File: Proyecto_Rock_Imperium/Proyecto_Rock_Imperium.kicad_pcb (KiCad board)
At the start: 2 copper layers, 53.3 x 58.4 mm, 20 parts, among them Q1 2N3904, Q2 2N3904, SW1 SW_SPDT

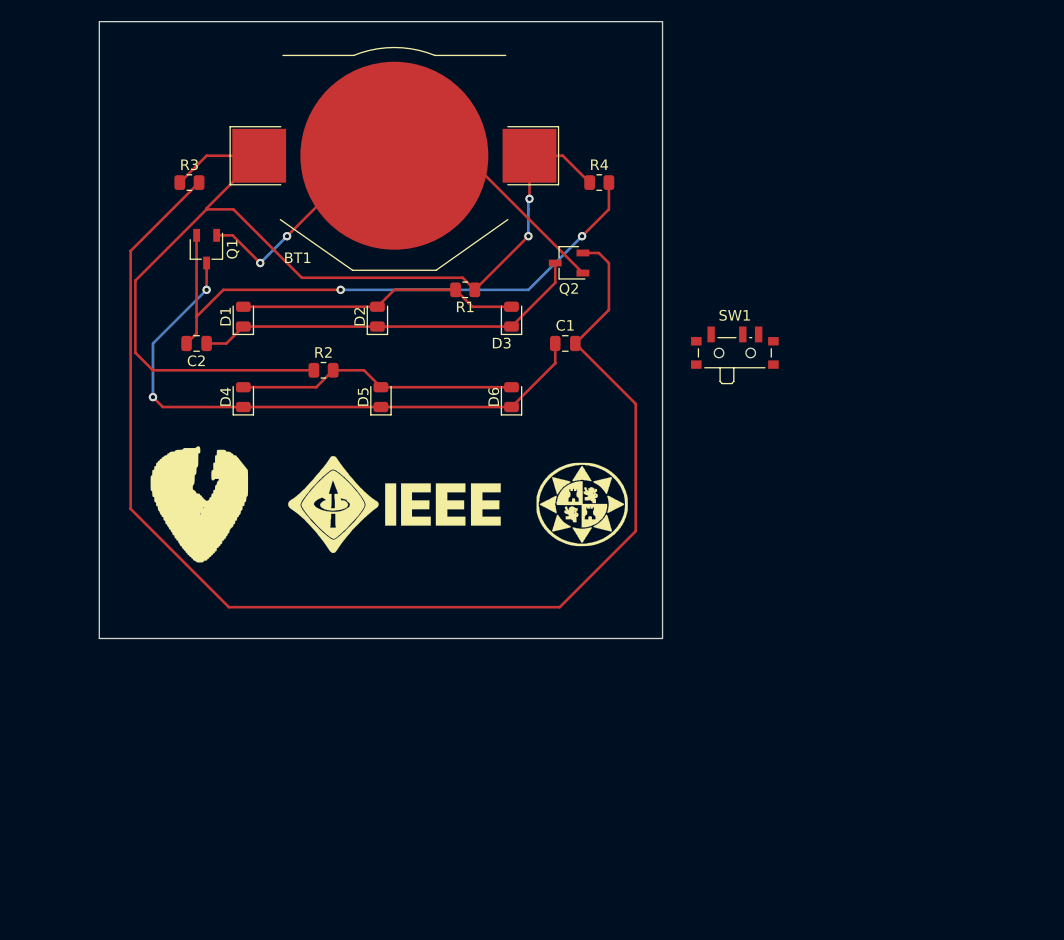
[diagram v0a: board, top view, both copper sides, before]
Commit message: terminado a falta de revision
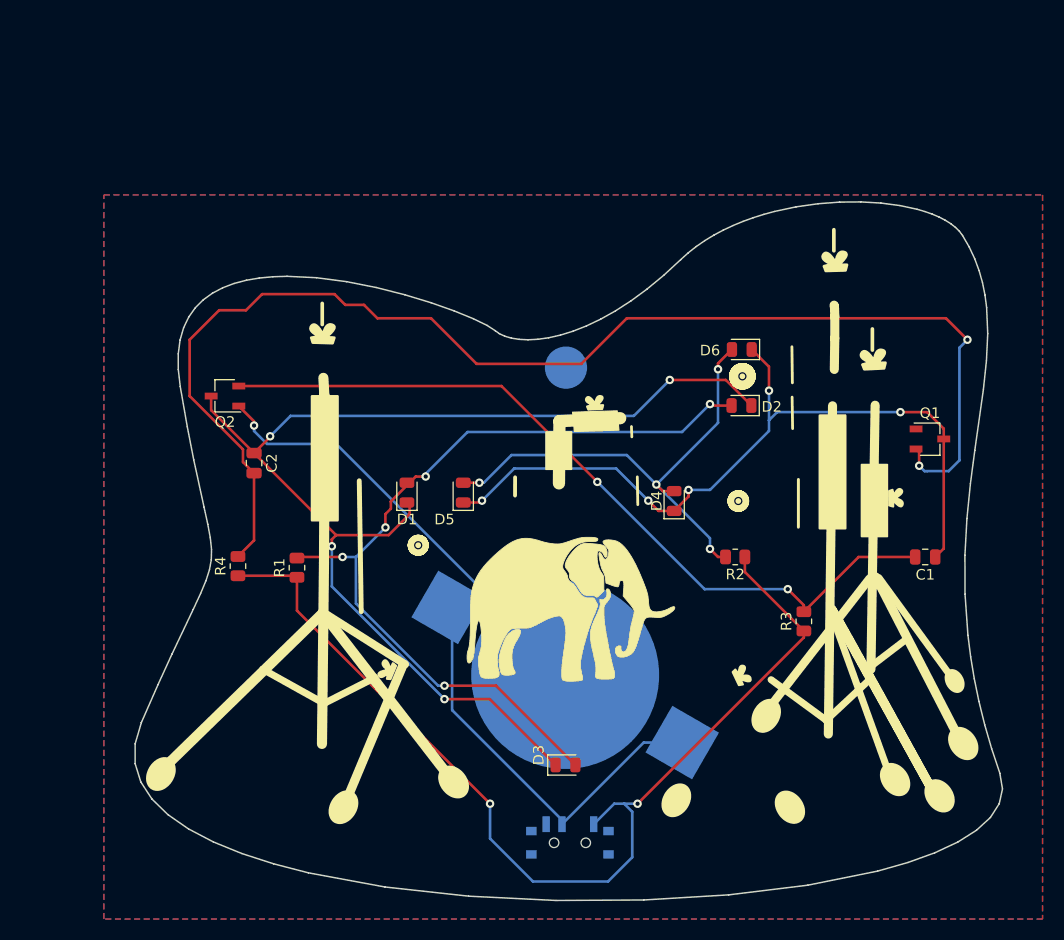
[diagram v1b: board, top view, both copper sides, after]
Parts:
- removed Ref**: Val**, proyecto_rock:RoCkImPeRiUm
- removed Ref**: Val**, proyecto_rock:IEEE2
- removed Ref**: Val**, proyecto_rock:UPCT2
- removed Ref**: Val**, proyecto_rock:UPCT
- added REF**: TestPoint_Pad_D4.0mm, TestPoint:TestPoint_Pad_D4.0mm, B.Cu at (156.0, 78.5)
- BT1, SW1: moved to B.Cu
- moved R3 71.5 mm to (178.5, 102.5), turned to 90 degrees
- moved Q1 70.8 mm to (190.4, 85.2), turned to 0 degrees
- moved BT1 51.8 mm to (155.9, 107.6), turned to 150 degrees
- moved R4 49.9 mm to (124.9, 97.3), turned to 90 degrees
- moved SW1 48.9 mm to (156.3, 123.2), turned to 180 degrees
- moved R2 42.8 mm to (172.0, 96.4), turned to 180 degrees
- moved D3 42.8 mm to (155.9, 116.1), turned to 0 degrees
- moved D4 42.0 mm to (166.2, 91.1)
- moved C1 39.6 mm to (190.0, 96.4), turned to 180 degrees
- moved D2 35.5 mm to (172.6, 82.1), turned to 180 degrees
- moved Q2 34.9 mm to (123.7, 81.2)
- moved R1 30.8 mm to (130.5, 97.4), turned to 90 degrees
- moved D1 22.8 mm to (140.9, 90.3)
- moved D6 22.3 mm to (172.6, 76.8), turned to 180 degrees
- moved C2 12.6 mm to (126.4, 87.5), turned to -90 degrees
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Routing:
- net (no net): track 99.8 -> 0.00 mm, vias 2 -> 0
- net /sw_on: track 0.00 -> 96.6 mm, vias 0 -> 2
- net /k_b: track 37.3 -> 111.2 mm, vias 0 -> 4
- net /chr_a: track 56.4 -> 122.4 mm
- net /leds_b: track 26.7 -> 80.1 mm, vias 0 -> 5
- net /chr_b: track 120.2 -> 75.4 mm, vias 0 -> 2
- net +3V0: track 0.00 -> 39.6 mm
- net /leds_a: track 26.7 -> 48.0 mm, vias 0 -> 4
- net /k_a: track 56.9 -> 73.6 mm, vias 2 -> 5
- net GND: track 44.6 -> 42.1 mm, vias 2 -> 1
- added copper zone on B.Cu, net GND
- added copper zone on F.Cu, net GND
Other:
- board size 53.3 x 58.4 mm -> 82.1 x 66.2 mm

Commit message: terminado. Pendiente revision y pulir bateria
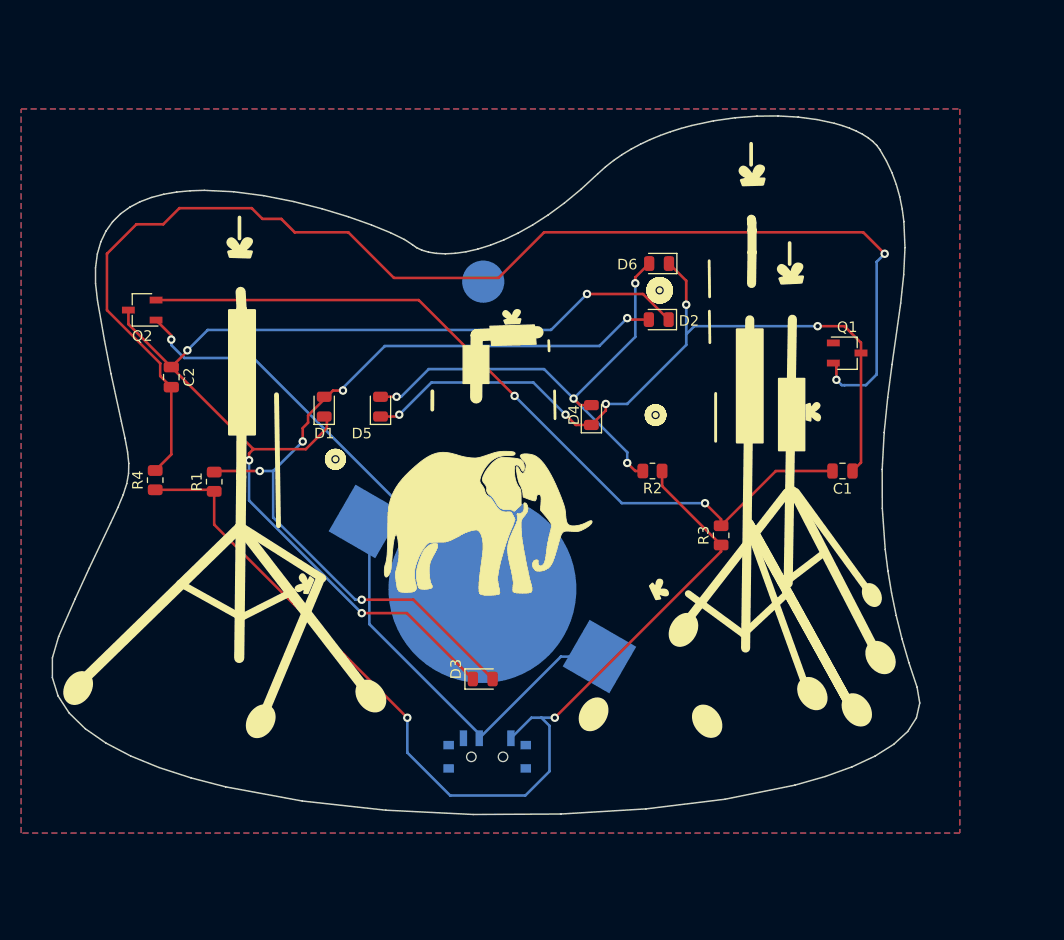
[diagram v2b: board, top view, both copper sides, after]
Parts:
- moved C1 11.3 mm to (182.1, 88.3)
- moved C2 11.3 mm to (118.6, 79.4)
- moved D3 11.3 mm to (148.1, 108.0)
- moved D4 11.3 mm to (158.4, 83.0)
- moved Q1 11.3 mm to (182.6, 77.1)
- moved Q2 11.3 mm to (115.8, 73.0)
- moved R1 11.3 mm to (122.6, 89.3)
- moved R2 11.3 mm to (164.1, 88.3)
- moved R4 11.3 mm to (117.1, 89.1)
- moved D1 11.3 mm to (133.1, 82.2)
- moved D5 11.3 mm to (138.4, 82.2)
- moved BT1 11.3 mm to (148.0, 99.5)
- moved R3 11.3 mm to (170.6, 94.4)
- moved REF** 11.3 mm to (148.1, 70.3)
- moved D2 11.3 mm to (164.7, 73.9)
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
